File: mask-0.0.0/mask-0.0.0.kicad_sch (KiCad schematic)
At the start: 20 parts, among them J1 Conn_02x05_Counter_Clockwise, J2 Conn_ARM_JTAG_SWD_10, Q1 IRLML2502, U1 NORA-B10x, U2 MCP1703A-3302_SOT23

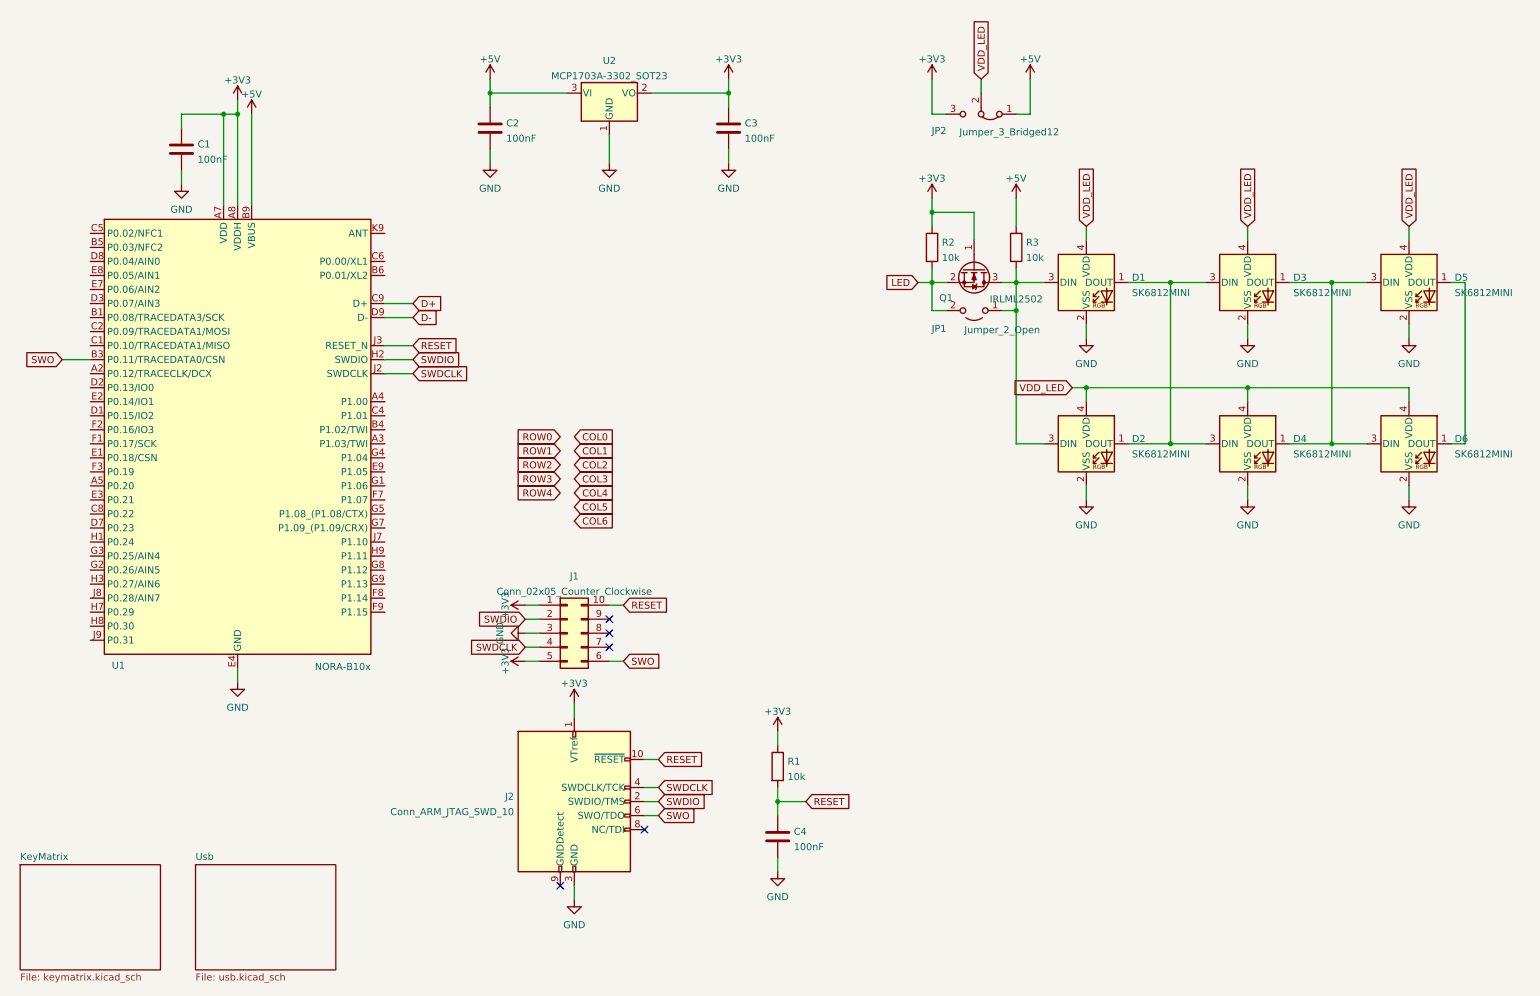
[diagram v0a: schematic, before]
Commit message: mask-0.0.0: begin of matrix routing
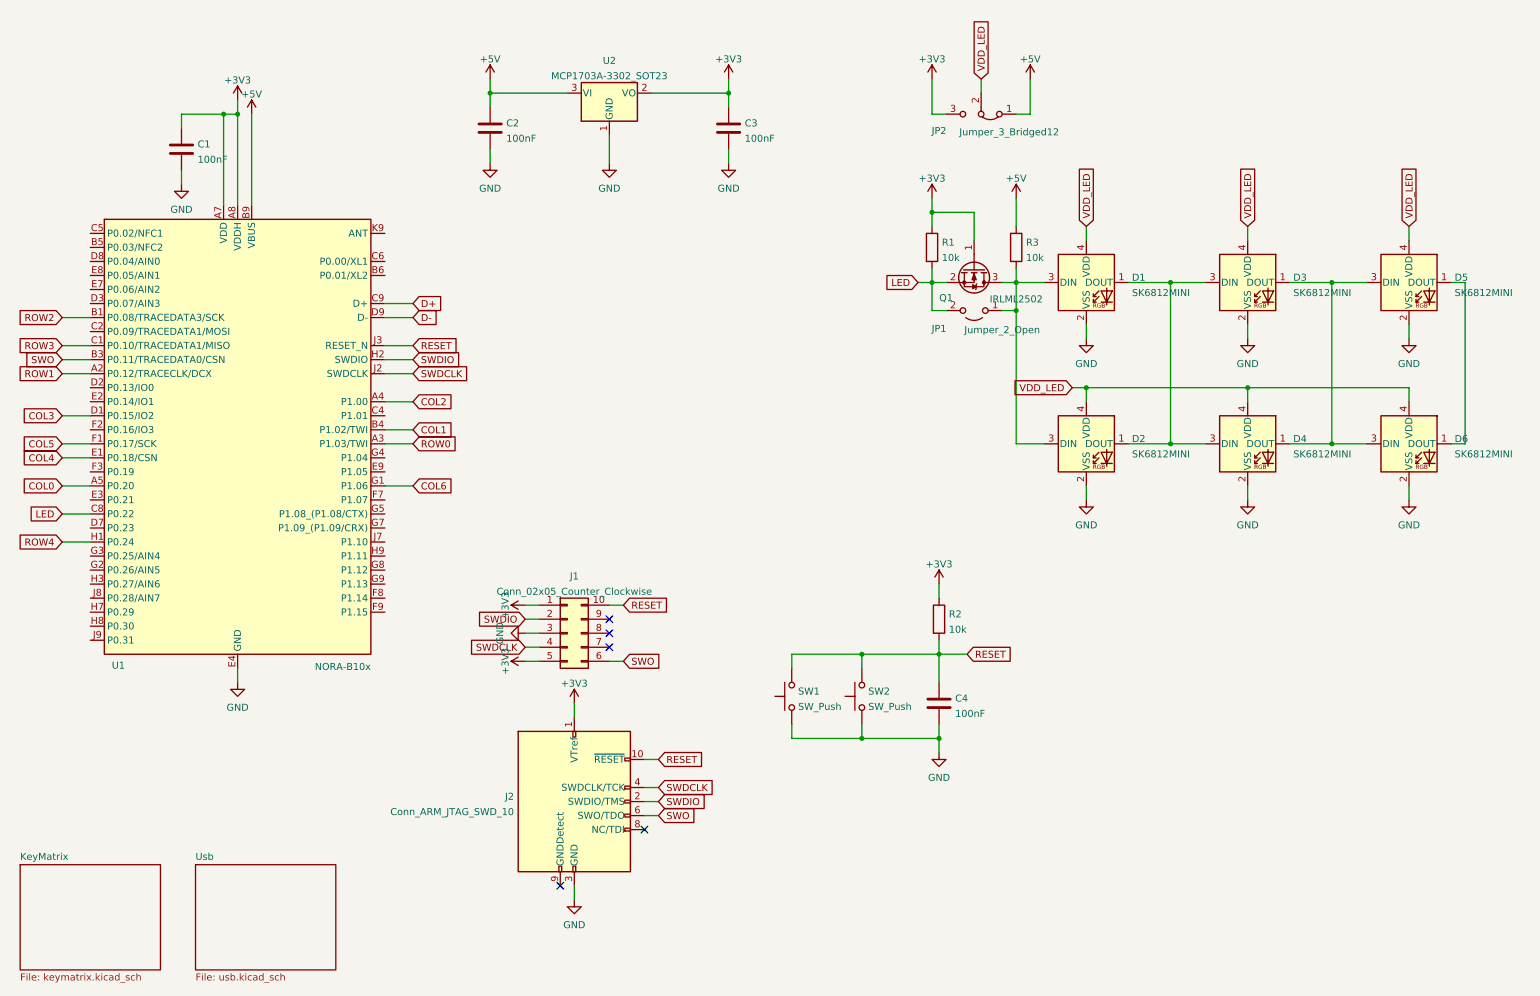
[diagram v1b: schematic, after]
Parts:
- added SW1, SW2: SW_Push, Button_Switch_SMD:SW_SPST_B3U-1000P, symbol Switch:SW_Push
- renumbered R2 to R1, R1 to R2
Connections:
- net COL0: now also U1.A5 (P0.20)
- net COL1: now also U1.B4 (P1.02/TWI)
- net COL2: now also U1.A4 (P1.00)
- net COL3: now also U1.D1 (P0.15/IO2)
- net COL4: now also U1.E1 (P0.18/CSN)
- net COL5: now also U1.F1 (P0.17/SCK)
- net COL6: now also U1.G1 (P1.06)
- net GND: now also SW1.1, SW2.1
- net LED: now also U1.C8 (P0.22)
- net RESET: now also SW1.2, SW2.2
- net ROW0: now also U1.A3 (P1.03/TWI)
- net ROW1: now also U1.A2 (P0.12/TRACECLK/DCX)
- net ROW2: now also U1.B1 (P0.08/TRACEDATA3/SCK)
- net ROW3: now also U1.C1 (P0.10/TRACEDATA1/MISO)
- net ROW4: now also U1.H1 (P0.24)
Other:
- moved on the sheet: C4, R2
